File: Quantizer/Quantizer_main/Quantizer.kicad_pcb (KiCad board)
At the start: 2 copper layers, 48.1 x 100.1 mm, 35 parts, among them J0 POWER, J1 OUT, J2 CV-IN, J3 TRIG OUT, J4 SLIDE IN, SW1 Rotary_Encoder, SW2 SLIDE SW, U1 MCP4726

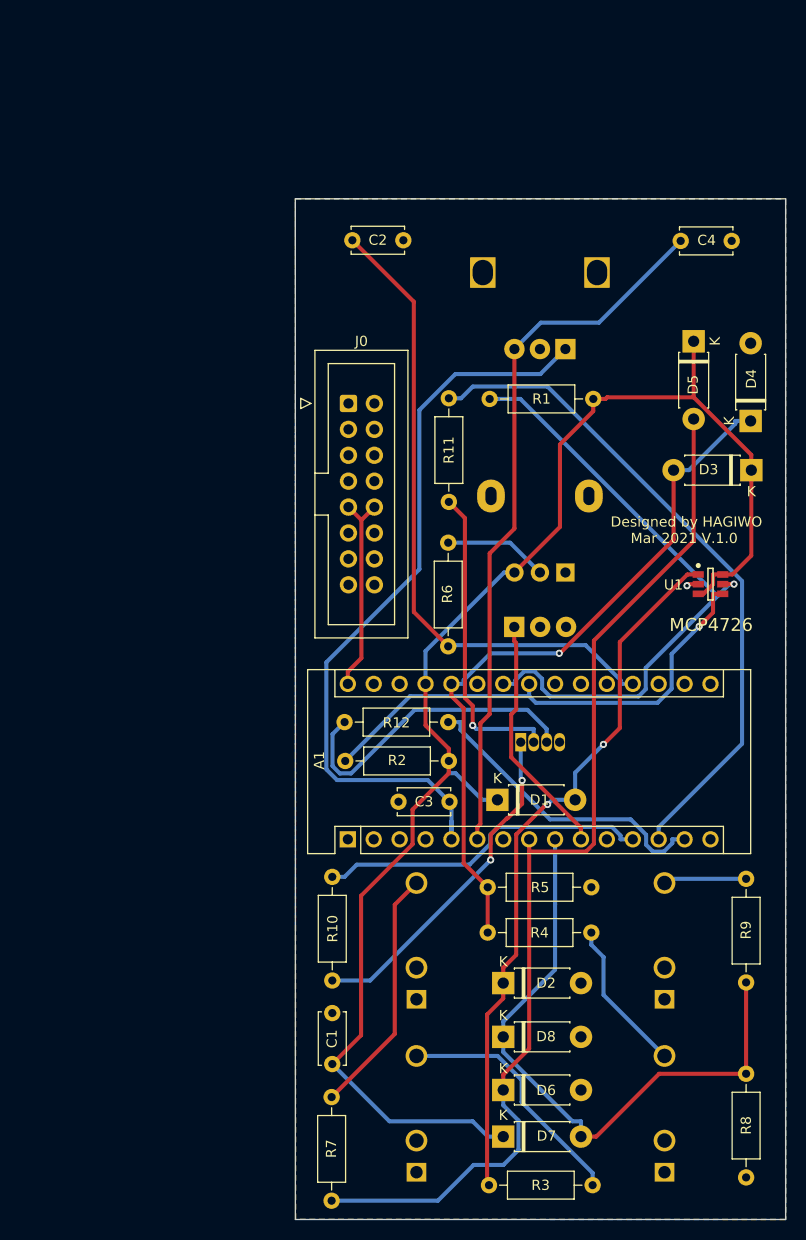
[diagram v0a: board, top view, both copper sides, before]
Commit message: correct
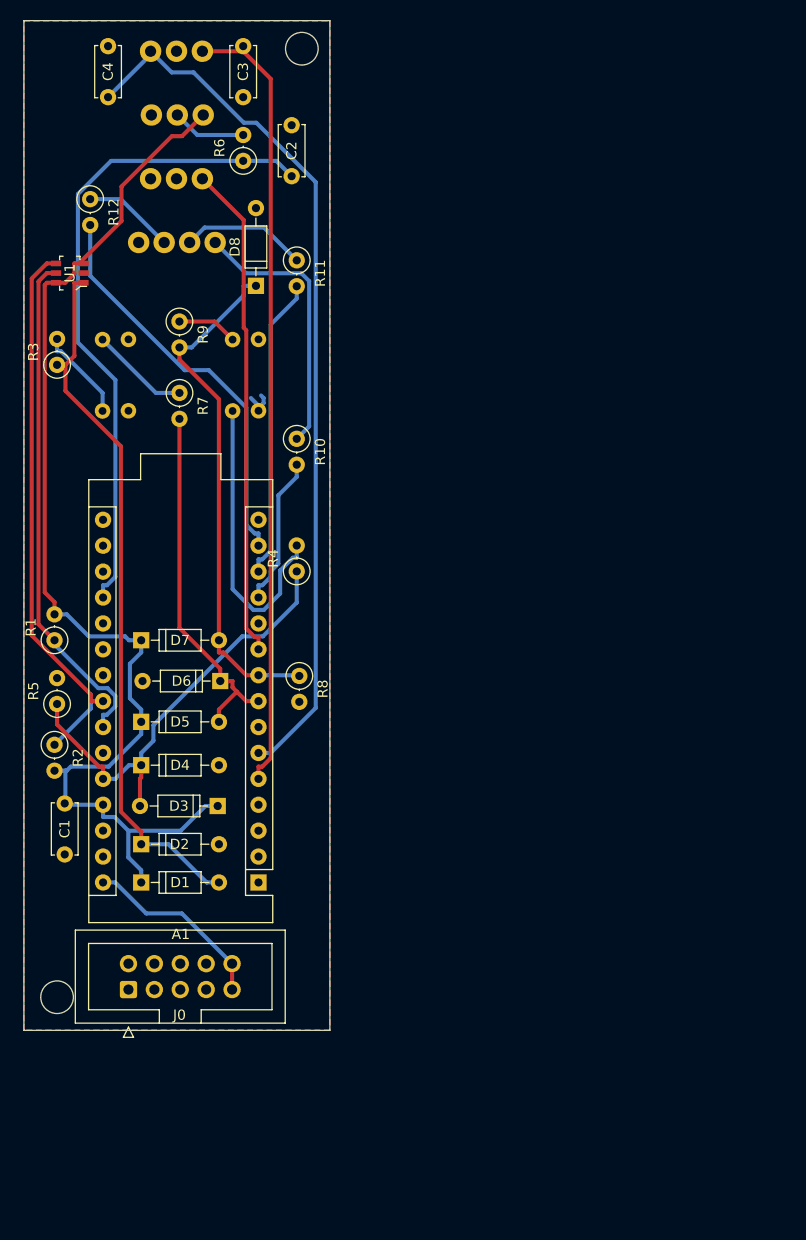
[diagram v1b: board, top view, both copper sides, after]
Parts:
- added REF1: MountingHole_3.2mm_M3, Mounting_Holes:MountingHole_3.2mm_M3, F.Cu at (87.2, 42.8)
- added REF2: MountingHole_3.2mm_M3, Mounting_Holes:MountingHole_3.2mm_M3, F.Cu at (63.2, 135.8)
- A1: footprint Module:Arduino_Nano -> Arduino:Arduino_Nano
- C1, C2, C3, C4: footprint Capacitor_THT:C_Disc_D5.0mm_W2.5mm_P5.00mm -> Capacitors_THT:C_Disc_D5.0mm_W2.5mm_P5.00mm
- D1, D2, D3, D4, D5, D6, D7, D8: footprint Diode_THT:D_DO-41_SOD81_P7.62mm_Horizontal -> Diodes_THT:D_DO-35_SOD27_P7.62mm_Horizontal
- D9: footprint LED_THT:LED_D5.0mm-4_RGB -> digikey-footprints:PinHeader_1x4_P2.5mm_Drill1.1mm
- J0: footprint Connector_IDC:IDC-Header_2x08_P2.54mm_Vertical -> Connector_IDC:IDC-Header_2x05_P2.54mm_Vertical
- J1, J2, J3, J4: footprint Connector_Audio:Jack_3.5mm_QingPu_WQP-PJ398SM_Vertical_CircularHoles -> digikey-footprints:PinHeader_1x2_P2.54mm
- R1, R10, R11, R12, R2, R3, R4, R5, R6, R7, R8, R9: footprint Resistor_THT:R_Axial_DIN0207_L6.3mm_D2.5mm_P10.16mm_Horizontal -> Resistors_THT:R_Axial_DIN0207_L6.3mm_D2.5mm_P2.54mm_Vertical
- RV1: footprint Potentiometer_THT:Potentiometer_Alpha_RD901F-40-00D_Single_Vertical -> digikey-footprints:PinHeader_1x3_P2.54_Drill1.1mm
- SW1: footprint Rotary_Encoder:RotaryEncoder_Alps_EC12E_Vertical_H20mm -> digikey-footprints:PinHeader_1x3_P2.54_Drill1.1mm
- SW2: footprint digikey-footprints:Switch_Toggle_ATE1D-2M3-10-Z -> digikey-footprints:PinHeader_1x3_P2.54_Drill1.1mm
- U1: footprint digikey-footprints:Microchip-MCP4726A0T-E_CH-Level_B -> digikey-footprints:SOT-23-6
- moved R3 90.9 mm to (63.2, 73.8), turned to 90 degrees
- moved J2 84.6 mm to (83.0, 78.2), turned to 180 degrees
- moved J1 79.8 mm to (70.2, 78.2), turned to 180 degrees
- moved R9 77.9 mm to (75.2, 69.5)
- moved D8 77.5 mm to (82.8, 66.0), turned to 90 degrees
- moved C3 76.8 mm to (81.5, 42.5), turned to 270 degrees
- moved J4 76.0 mm to (83.0, 71.2), turned to 180 degrees
- moved R7 70.6 mm to (75.2, 76.5)
- moved J3 70.6 mm to (70.2, 71.2), turned to 180 degrees
- moved U1 69.8 mm to (64.5, 64.8), turned to 90 degrees
- moved D4 68.6 mm to (71.5, 113.0), turned to 0 degrees
- moved D5 65.8 mm to (71.5, 108.8), turned to 0 degrees
- moved D3 61.8 mm to (79.0, 117.0)
- moved J0 61.4 mm to (70.2, 135.0), turned to 90 degrees
- moved RV1 60.5 mm to (72.5, 49.2), turned to 0 degrees
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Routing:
- net Net-(A1-Pad8): track 105.5 -> 36.0 mm
- net Net-(A1-Pad13): track 66.4 -> 29.8 mm
- net 5V: track 146.2 -> 114.4 mm
- net Net-(A1-Pad26): track 70.8 -> 44.3 mm, vias 1 -> 0
- net Net-(A1-Pad10): track 24.6 -> 48.6 mm
- net Net-(D9-Pad3): track 30.7 -> 9.01 mm
- net Net-(A1-Pad9): track 69.0 -> 50.9 mm
- net Net-(A1-Pad12): track 32.7 -> 14.8 mm
- net Net-(D9-Pad2): track 30.3 -> 12.4 mm, vias 1 -> 0
- net Net-(A1-Pad6): track 70.9 -> 86.6 mm
- net Net-(J1-PadT): track 24.5 -> 9.13 mm
- net Net-(J3-PadT): track 24.4 -> 9.71 mm
- net Net-(J2-PadT): track 15.1 -> 29.3 mm
- net Net-(A1-Pad24): track 62.2 -> 50.1 mm, vias 1 -> 0
- net Net-(A1-Pad14): track 30.2 -> 39.9 mm
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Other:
- board size 48.1 x 100.1 mm -> 30 x 99 mm
- board text removed: "Designed by HAGIWO Mar 2021 V.1.0"
